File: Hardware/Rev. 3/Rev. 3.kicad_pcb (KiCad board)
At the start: 4 copper layers, 25.5 x 32.7 mm, 13 parts, among them U1 MCP73831-2-OT, U3 W25Q128JVS

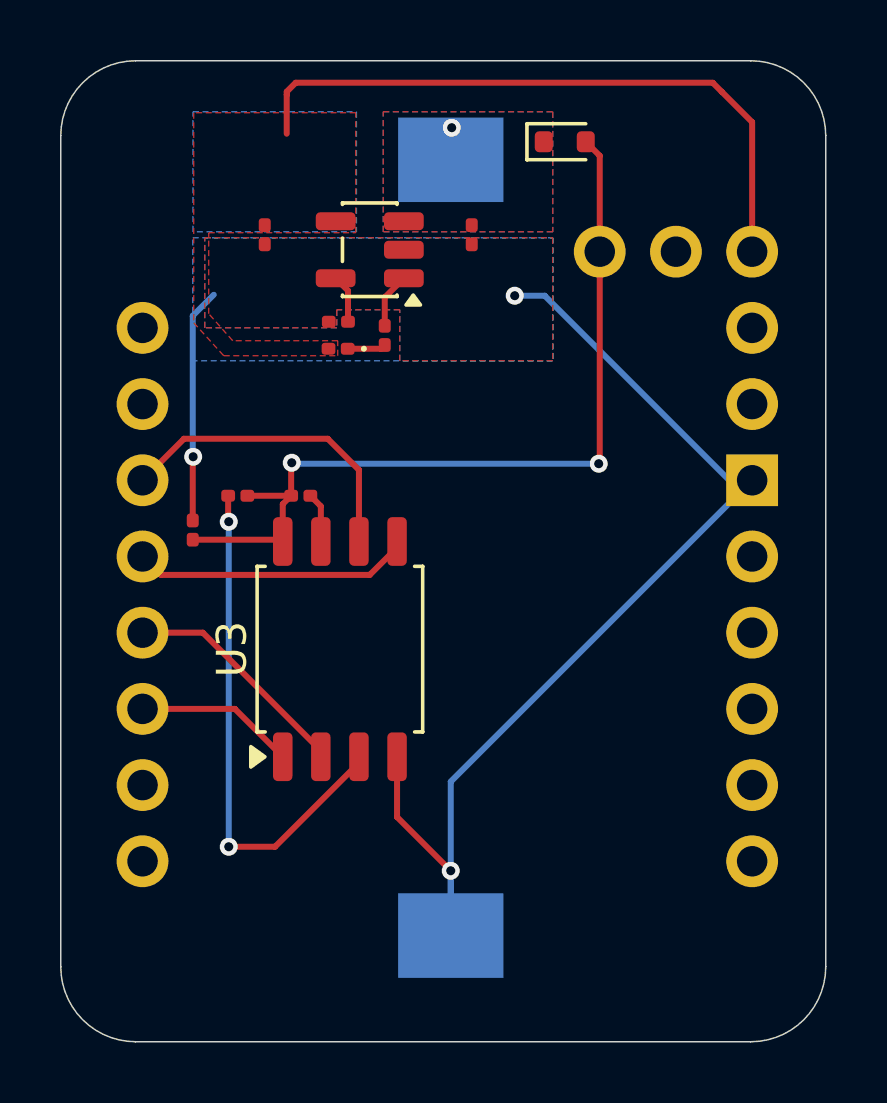
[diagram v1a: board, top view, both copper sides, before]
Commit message: Week 3
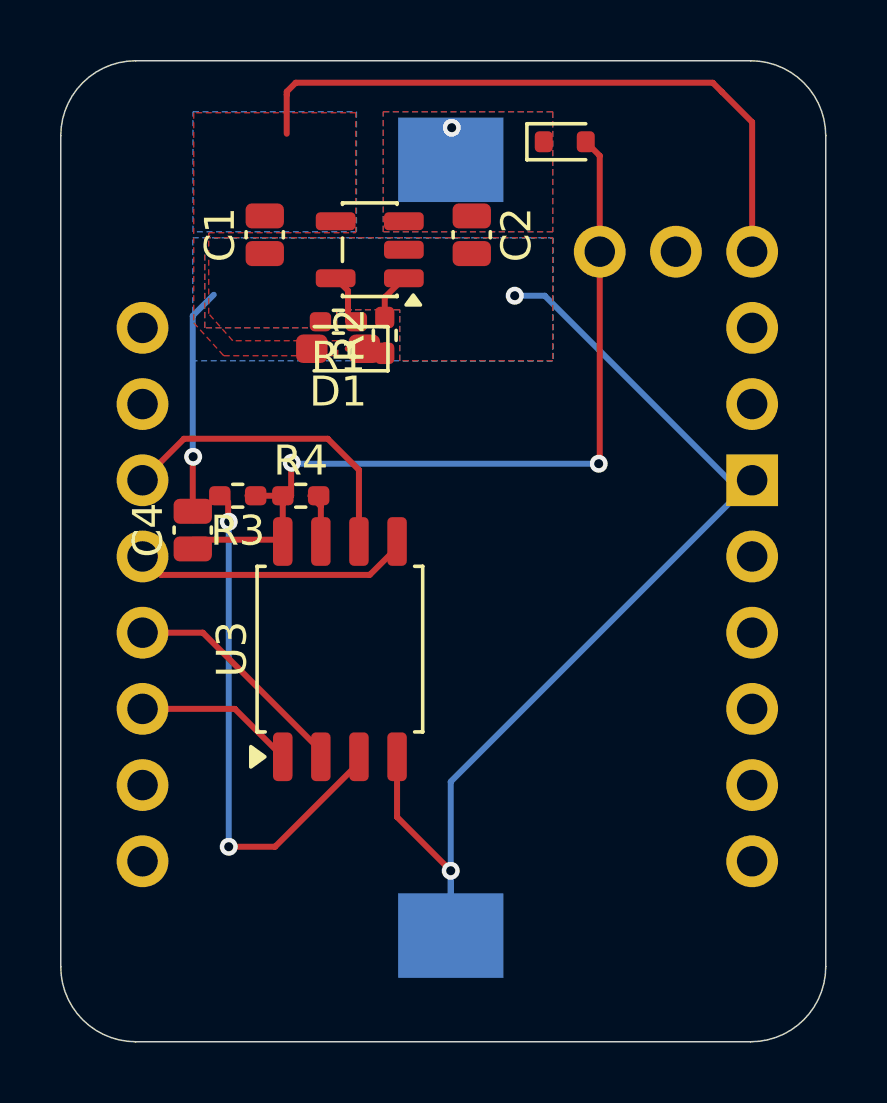
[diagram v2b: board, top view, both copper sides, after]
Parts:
- C1, C2, C4: footprint Capacitor_SMD:C_0201_0603Metric -> Capacitor_SMD:C_0504_1310Metric_Pad0.83x1.28mm_HandSolder
- D1: footprint Diode_SMD:D_0201_0603Metric -> Diode_SMD:D_0603_1608Metric_Pad1.05x0.95mm_HandSolder
- R1, R2, R3, R4: footprint Resistor_SMD:R_0201_0603Metric -> Resistor_SMD:R_0402_1005Metric_Pad0.72x0.64mm_HandSolder
